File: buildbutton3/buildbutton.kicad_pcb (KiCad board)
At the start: 2 copper layers, 34 x 36 mm, 17 parts, among them J1 BATTERY, J2 IO0, J3 BUTTON, J4 LED, J5 USB, Q1 IRLIZ44N, U1 S7V8F3, U2 U3V12F9, U3 ESP32_DATA, U4 ESP_UART

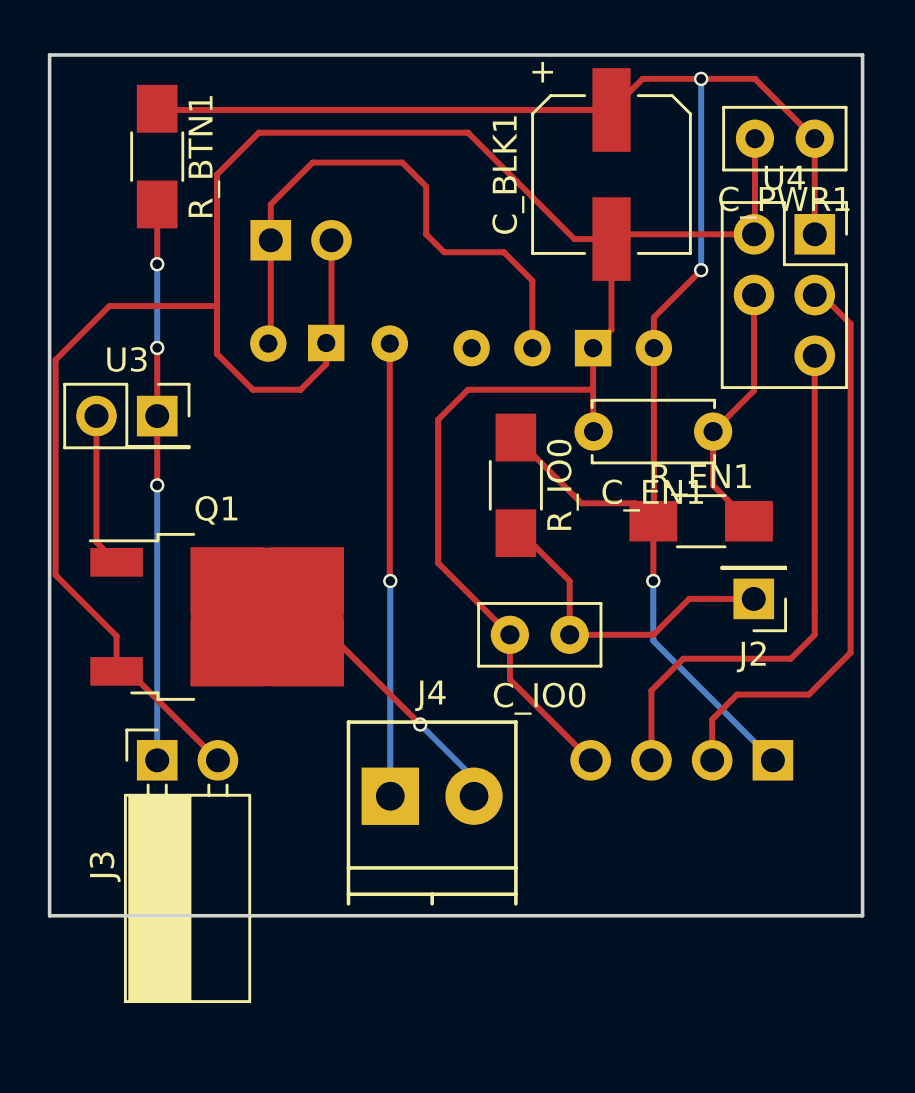
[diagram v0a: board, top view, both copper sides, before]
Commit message: BuildButton v3
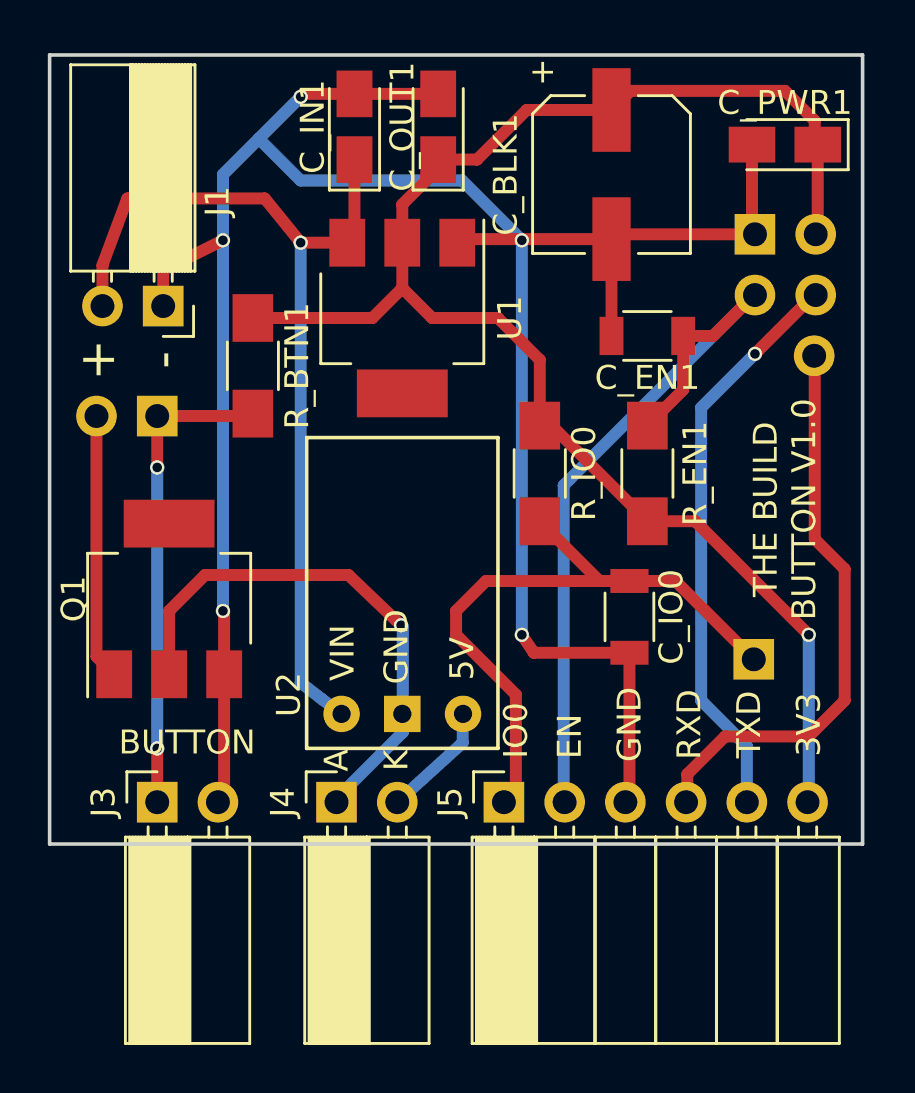
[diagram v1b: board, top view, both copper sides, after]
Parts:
- added C_IN1: 10uF, Capacitors_Tantalum_SMD:CP_Tantalum_Case-A_EIA-3216-18_Reflow, F.Cu at (79.8, 71.0)
- added C_OUT1: 10uF, Capacitors_Tantalum_SMD:CP_Tantalum_Case-A_EIA-3216-18_Reflow, F.Cu at (83.2, 71.0)
- C_EN1: value 1nF -> 2.2nF; footprint Capacitors_THT:C_Disc_D5.0mm_W2.5mm_P5.00mm -> Capacitors_SMD:C_1206
- C_IO0: value 1nF -> 2.2nF; footprint Capacitors_THT:C_Disc_D5.0mm_W2.5mm_P2.50mm -> Capacitors_SMD:C_1206
- C_PWR1: footprint Capacitors_THT:C_Disc_D5.0mm_W2.5mm_P2.50mm -> Capacitors_Tantalum_SMD:CP_Tantalum_Case-A_EIA-3216-18_Reflow
- J1: moved to F.Cu
- J2: footprint Socket_Strips:Socket_Strip_Straight_1x01_Pitch2.54mm -> Socket_Strips:Socket_Strip_Straight_2x01_Pitch2.54mm; moved to B.Cu
- J4: footprint TerminalBlocks_Phoenix:TerminalBlock_Phoenix_PT-3.5mm_2pol -> Socket_Strips:Socket_Strip_Angled_1x02_Pitch2.54mm
- J5: value USB -> PROG; footprint Socket_Strips:Socket_Strip_Angled_1x04_Pitch2.54mm -> Socket_Strips:Socket_Strip_Angled_1x06_Pitch2.54mm; moved to F.Cu
- Q1: value IRLIZ44N -> IRLL014N; footprint TO_SOT_Packages_SMD:TO-252-2 -> TO_SOT_Packages_SMD:SOT-223
- U1: value S7V8F3 -> LM1117-3.3; footprint pololu:S7V8F3 -> TO_SOT_Packages_SMD:SOT-223; moved to F.Cu
- U2: value U3V12F9 -> U3V12F5; footprint pololu:U3V12F9 -> U3V12F9; moved to F.Cu
- U3, U4: moved to B.Cu
- moved U1 16.5 mm to (81.8, 79.0), turned to 270 degrees
- moved J5 11.4 mm to (86.0, 99.2)
- moved R_BTN1 9.62 mm to (75.5, 81.0)
- moved U2 8.08 mm to (77.8, 84.0), turned to 270 degrees
- moved J1 5.27 mm to (71.8, 78.5)
- moved C_EN1 4.85 mm to (92.0, 79.8)
- moved R_EN1 3.01 mm to (92.0, 85.5), turned to 90 degrees
- moved C_IO0 2.61 mm to (91.2, 91.5), turned to 270 degrees
- moved J2 2.53 mm to (96.5, 93.3)
- moved U4 2.50 mm to (96.5, 75.5), turned to 180 degrees
- moved J4 2.26 mm to (79.0, 99.2), turned to 90 degrees
- moved Q1 2.14 mm to (72.0, 90.8), turned to 90 degrees
- moved J3 1.75 mm to (71.5, 99.2)
- moved C_PWR1 1.27 mm to (97.8, 71.8)
- moved R_IO0 1.12 mm to (87.5, 85.5)
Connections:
- net 9V renamed Net-(J4-Pad1)
- C_IO0 pad 1: Net-(C_IO0-Pad1) -> IO0
- J2 pad 1: Net-(C_IO0-Pad1) -> IO0
- R_IO0 pad 2: Net-(C_IO0-Pad1) -> IO0
- U1 pad 1: VCC -> GND
- U1 pad 2: GND -> 3V3
- U1 pad 3: 3V3 -> VCC
- U2 pad 2: GND -> Net-(J4-Pad2)
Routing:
- net IO0: track 0.00 -> 27.2 mm
- net EN: track 10.8 -> 32.6 mm
- net VCC: track 23.6 -> 39.3 mm, vias 0 -> 1
- net Net-(J4-Pad1): track 18.9 -> 4.83 mm, vias 1 -> 0
- net Net-(C_IO0-Pad1): track 13.6 -> 0.00 mm
- net Net-(J4-Pad2): track 12.2 -> 22.4 mm
- net GND: track 107.5 -> 102.1 mm, vias 0 -> 5
- net 3V3: track 71.7 -> 66.4 mm, vias 3 -> 1
- net Net-(Q1-Pad1): track 6.47 -> 11.1 mm
- net Net-(J3-Pad1): track 23.2 -> 20.2 mm, vias 3 -> 2
- net Net-(J5-Pad3): track 22.4 -> 24.0 mm
- net Net-(J5-Pad2): track 24.4 -> 24.0 mm, vias 0 -> 1
- added copper zone on F.Cu, net 3V3
- added copper zone on B.Cu, net GND
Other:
- board size 34 x 36 mm -> 34 x 33 mm
- net class Default: clearance 0.2 -> 0.6; trace_width 0.25 -> 0.5
- rule trace_clearance: 0.2 -> 0.6
- rule trace_min: 0.2 -> 0.5
- board text added: "+"
- board text added: "-"
- board text added: "3V3"
- board text added: "5V"
- board text added: "A"
- board text added: "BUTTON"
- board text added: "EN"
- board text added: "GND"
- board text added: "IO0"
- board text added: "K"
- board text added: "RXD"
- board text added: "THE BUILD BUTTON V1.0"
- board text added: "TXD"
- board text added: "VIN"
